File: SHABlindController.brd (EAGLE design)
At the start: 130.5 x 22 mm, 40 parts, among them IC1 SPARKCORE, IC2 HLKPM01, IC3 RXB1, Q1 2N7002, Q2 2N7002

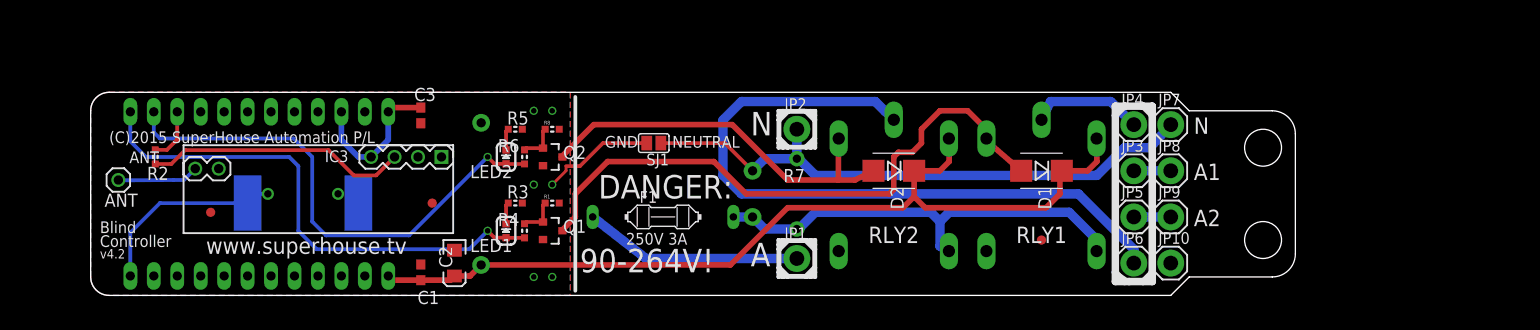
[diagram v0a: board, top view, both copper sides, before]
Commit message: Layout updates
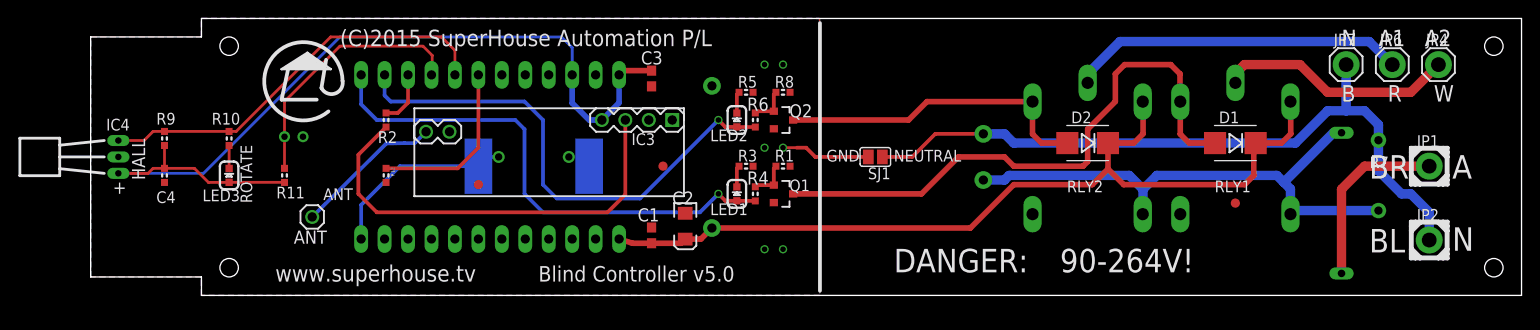
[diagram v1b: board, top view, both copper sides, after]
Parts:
- removed JP10: EARTH, freetronics-master-v1.1:1X01LARGE
- removed JP3, JP8: ACTIVE1, freetronics-master-v1.1:1X01LARGE
- removed JP5, JP9: ACTIVE2, freetronics-master-v1.1:1X01LARGE
- added C4: 100nF 0603, freetronics-master-v1.1:0603
- added IC4: AH180-PL-A, freetronics-jon:TO92FLATUP
- added LED3: ROTATE/GREEN, freetronics:LED-0603
- added R10: 1K 0603, freetronics-master-v1:0603
- added R11, R9: 10K 0603, freetronics-master-v1:0603
- added R12: 10K, freetronics:0603
- added S2: 2P-JST-PTH, freetronics-jon:JST-2MM-TH-RA
- moved F1 73.5 mm to (135.5, 10.0), flipped to the bottom, turned to 90 degrees
- moved JP2 69.5 mm to (145.0, 6.00)
- moved JP1 69.2 mm to (145.0, 14.0)
- moved R7 63.0 mm to (139.5, 13.0)
- moved JP6 35.3 mm to (141.0, 25.0)
- moved JP4 33.6 mm to (146.0, 25.0)
- moved FID2 29.2 mm to (42.0, 12.0)
- moved C1 25.3 mm to (60.8, 6.50)
- moved C2 25.3 mm to (64.4, 7.50)
- moved C3 25.3 mm to (60.8, 23.5)
- moved FID3 25.3 mm to (62.0, 14.0)
- moved IC1 25.3 mm to (42.0, 15.0)
- moved IC2 25.3 mm to (82.0, 15.0)
- moved IC3 25.3 mm to (63.0, 19.0)
- moved LED1 25.3 mm to (70.0, 11.0)
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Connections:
- removed net D3: IC1.P$4
- removed net D4: IC1.P$5
- removed net D5: IC1.P$6
- removed net EARTH: JP10.1
- removed net N$7: JP3.1, JP8.1
- removed net N$8: JP5.1, JP9.1
- new net D3_BUTTON: IC1.P$4, R11.1, S2.POS
- new net D4_ROTATE: IC1.P$5, IC4.3, R10.2, R9.1
- new net D5_TYPE: IC1.P$6, R12.1
- new net N$11: LED3.C, R10.1
- net GND: now also C4.2, IC4.2, R12.2, S2.NEG
- net VCC: now also C4.1, IC4.1, LED3.A, R11.2, R9.2
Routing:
- net VCC: track 16.4 -> 99.5 mm
- net D4_ROTATE: track 0.00 -> 44.4 mm
- net N$17: track 75.5 -> 36.5 mm
- net D3_BUTTON: track 0.00 -> 28.3 mm
- net D5_TYPE: track 0.00 -> 18.8 mm
- net N$135: track 28.5 -> 47.1 mm
- net NEUTRAL: track 63.6 -> 77.6 mm
- net N$14: track 12.3 -> 25.9 mm
- net ACTIVE: track 48.8 -> 59.2 mm
- net N$3: track 43.6 -> 34.6 mm
- net N$1: track 8.86 -> 16.1 mm
- net N$9: track 23.7 -> 19.7 mm
- net N$8: track 4.00 -> 0.00 mm
- net N$7: track 4.00 -> 0.00 mm
- net GND: track 12.4 -> 9.65 mm
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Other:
- board size 130.5 x 22 mm -> 155 x 30 mm
- board text added: "+"
- board text added: "B"
- board text added: "BL"
- board text added: "BR"
- board text added: "BUTTON"
- board text added: "Blind Controller v5.0"
- board text added: "HALL"
- board text added: "R"
- board text added: "ROTATE"
- board text added: "W"
- board text removed: "2 x 330R 0603 3 x 1K 0603 2 x 10K 0603 2 x 1N4004 SMA 2 x 1uF 0603 1 x 10uF 6.3V TANT 2 x 2N7002 2 x GREEN LED"
- board text removed: "Blind"
- board text removed: "Controller"
- board text removed: "v4.2"
